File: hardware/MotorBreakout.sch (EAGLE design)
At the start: 1 part

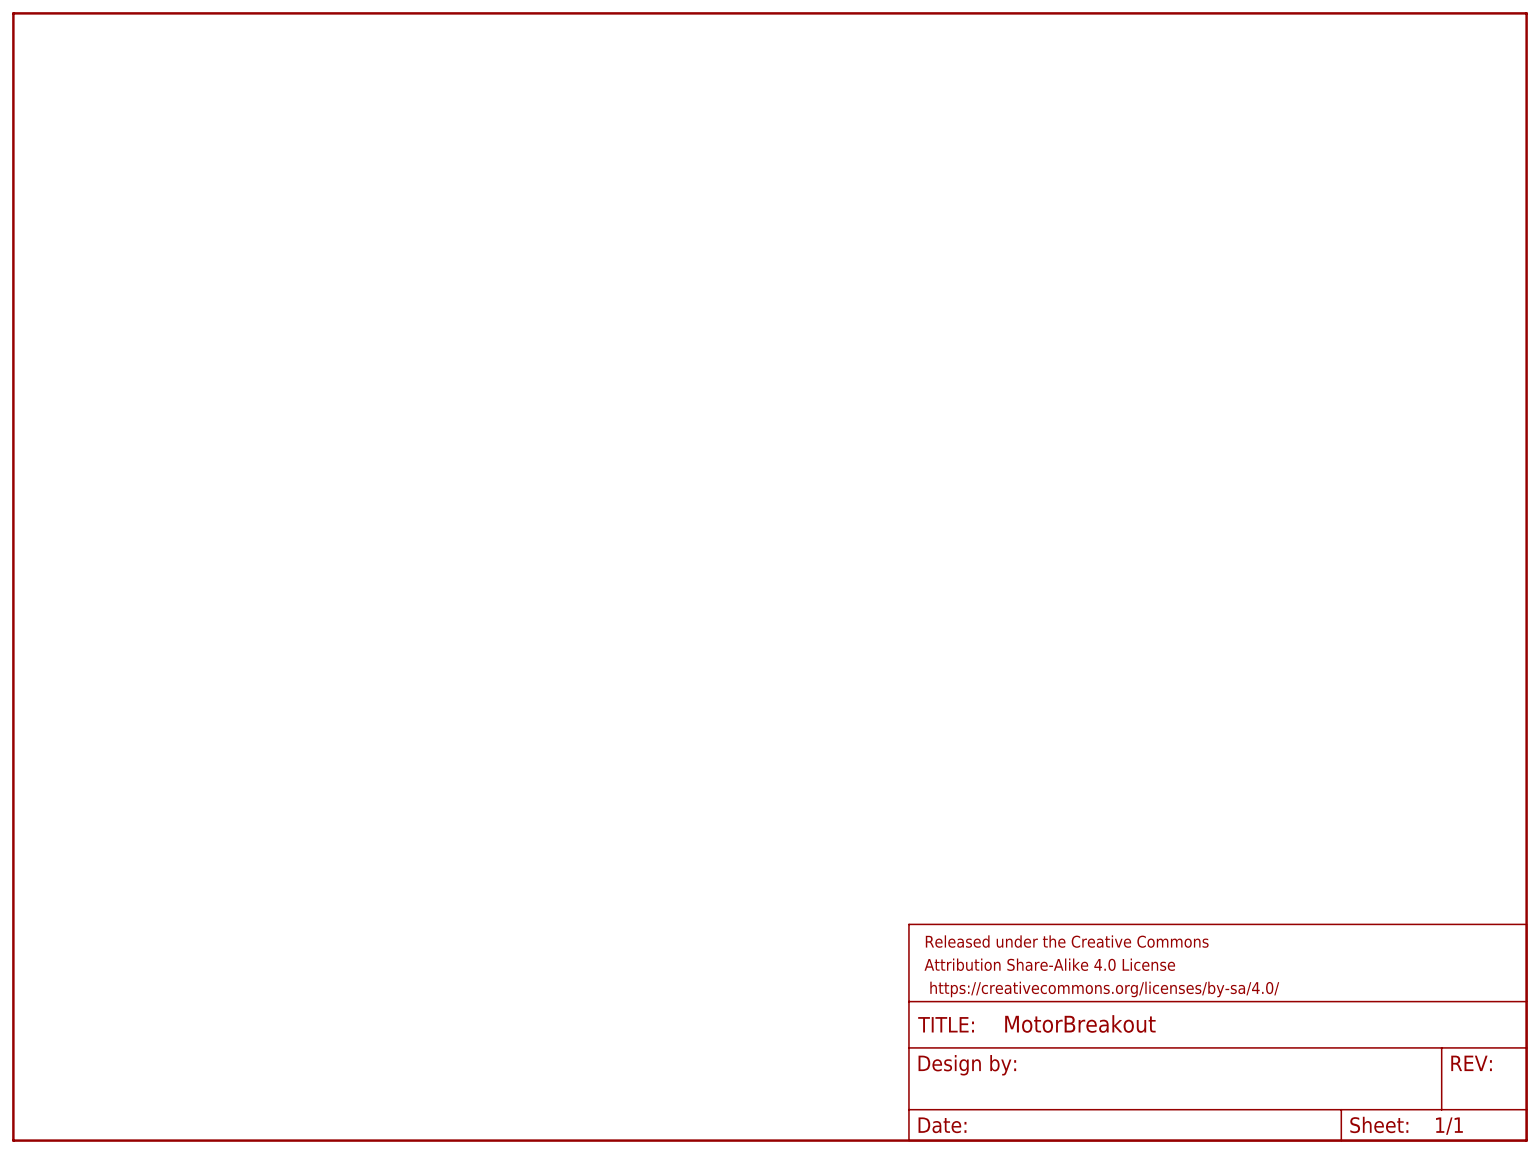
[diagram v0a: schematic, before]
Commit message: Basic breakout complete.y
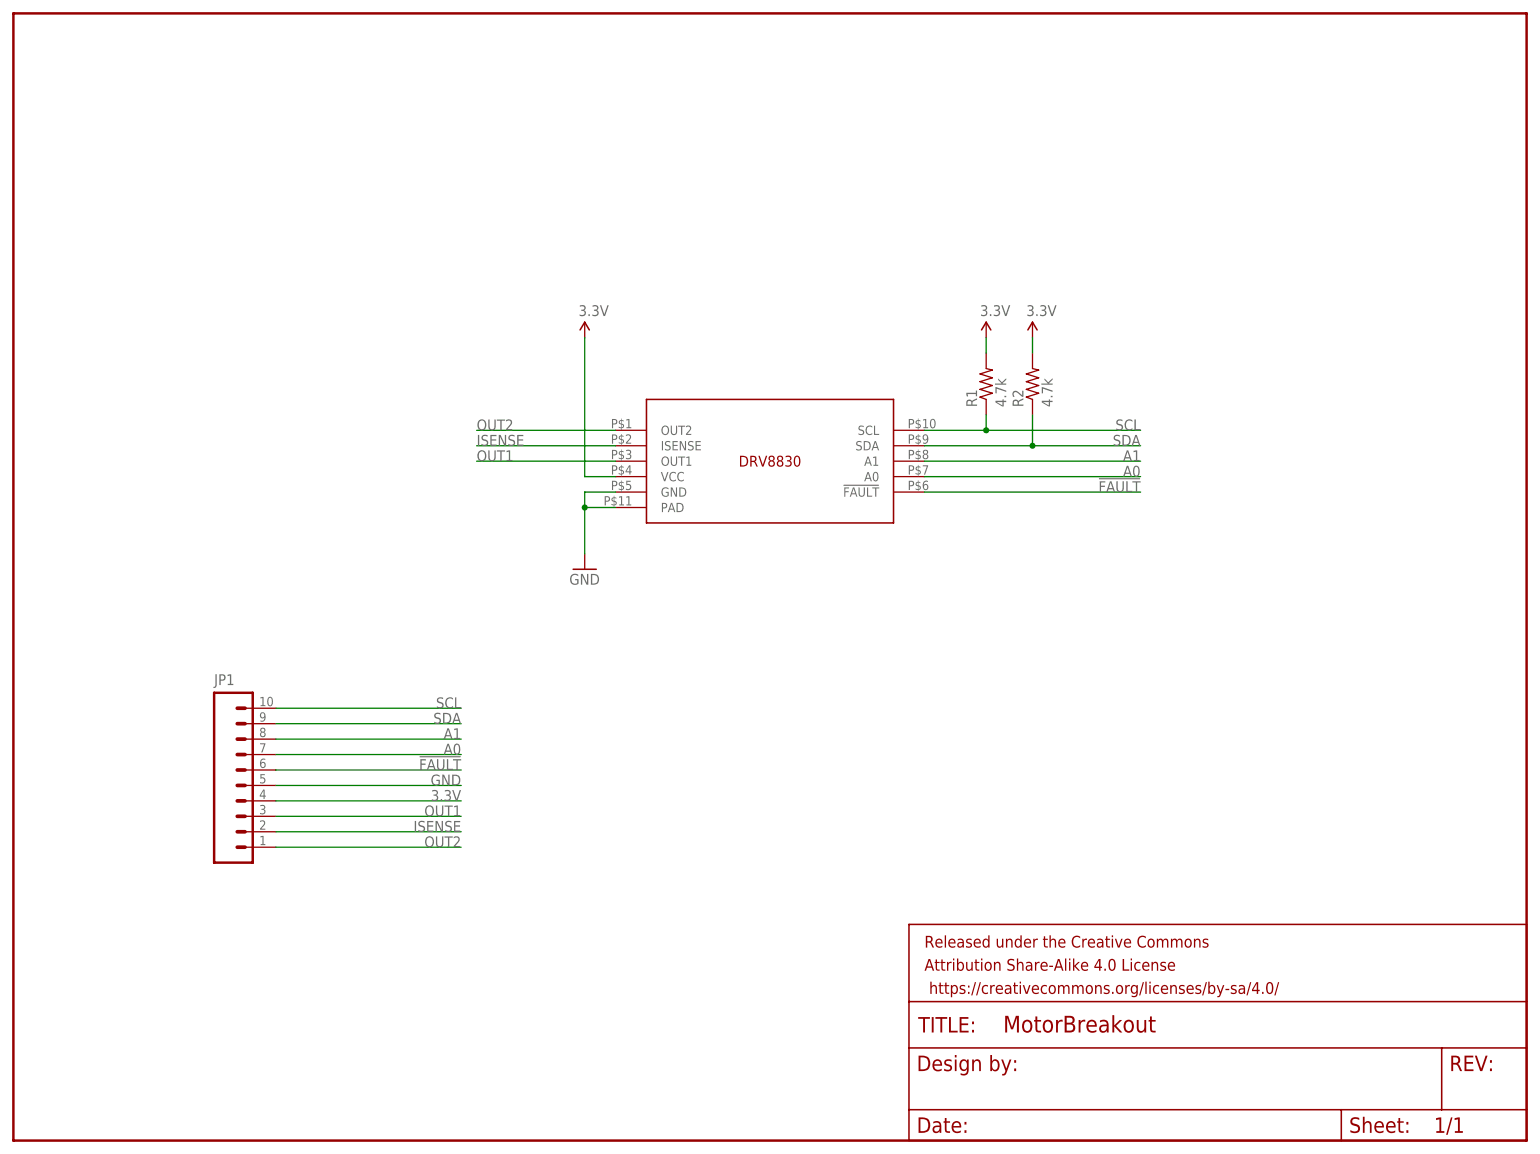
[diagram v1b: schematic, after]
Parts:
- added JP1: (no value), SparkFun-Connectors:M10LOCK_LONGPADS
- added R1, R2: 4.7k, SparkFun-Resistors:RESISTOR0402
- added U$1: DRV8830, DRV8830:DRV8830
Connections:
- new net !FAULT: JP1.6, U$1.!FAULT
- new net 3.3V: JP1.4, R1.2, R2.2, U$1.VCC
- new net A0: JP1.7, U$1.A0
- new net A1: JP1.8, U$1.A1
- new net GND: JP1.5, U$1.GND, U$1.PAD
- new net ISENSE: JP1.2, U$1.ISENSE
- new net OUT1: JP1.3, U$1.OUT1
- new net OUT2: JP1.1, U$1.OUT2
- new net SCL: JP1.10, R1.1, U$1.SCL
- new net SDA: JP1.9, R2.1, U$1.SDA
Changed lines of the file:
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@@
 <layer number="113" name="IDFDebug" color="4" fill="1" visible="yes" active="yes"/>
 <layer number="116" name="Patch_BOT" color="9" fill="4" visible="yes" active="yes"/>
+<layer number="118" name="Rect_Pads" color="7" fill="1" visible="yes" active="yes"/>
 <layer number="121" name="_tsilk" color="7" fill="1" visible="yes" active="yes"/>
 <layer number="122" name="_bsilk" color="7" fill="1" visible="yes" active="yes"/>
@@
 <parts>
 <part name="FRAME1" library="SparkFun-Aesthetics" deviceset="FRAME-LETTER" device="NO_PACKAGE"/>
+<part name="U$1" library="DRV8830" deviceset="DRV8830" device=""/>
+<part name="GND1" library="SparkFun-Aesthetics" deviceset="GND" device=""/>
+<part name="SUPPLY1" library="SparkFun-Aesthetics" deviceset="3.3V" device=""/>
+<part name="JP1" library="SparkFun-Connectors" deviceset="M10" device="LOCK_LONGPADS"/>
+<part name="SUPPLY2" library="SparkFun-Aesthetics" deviceset="3.3V" device=""/>
+<part name="SUPPLY3" library="SparkFun-Aesthetics" deviceset="3.3V" device=""/>
+<part name="R1" library="SparkFun-Resistors" deviceset="RESISTOR" device="0402" value="4.7k"/>
+<part name="R2" library="SparkFun-Resistors" deviceset="RESISTOR" device="0402" value="4.7k"/>
 </parts>
 <sheets>
@@
 <instance part="FRAME1" gate="G$1" x="0" y="0"/>
 <instance part="FRAME1" gate="V" x="147.32" y="0"/>
+<instance part="U$1" gate="G$1" x="124.46" y="111.76"/>
+<instance part="GND1" gate="1" x="93.98" y="93.98"/>
+<instance part="SUPPLY1" gate="G$1" x="93.98" y="132.08"/>
+<instance part="JP1" gate="G$1" x="33.02" y="66.04"/>
+<instance part="SUPPLY2" gate="G$1" x="160.02" y="132.08"/>
+<instance part="SUPPLY3" gate="G$1" x="167.64" y="132.08"/>
+<instance part="R1" gate="G$1" x="160.02" y="124.46" rot="R90"/>
+<instance part="R2" gate="G$1" x="167.64" y="124.46" rot="R90"/>
 </instances>
 <busses>
 </busses>
 <nets>
+<net name="3.3V" class="0">
+<segment>
+<pinref part="U$1" gate="G$1" pin="VCC"/>
+<pinref part="SUPPLY1" gate="G$1" pin="3.3V"/>
+<wire x1="99.06" y1="109.22" x2="93.98" y2="109.22" width="0.1524" layer="91"/>
+<wire x1="93.98" y1="109.22" x2="93.98" y2="132.08" width="0.1524" layer="91"/>
+</segment>
+<segment>
+<pinref part="JP1" gate="G$1" pin="4"/>
+<wire x1="43.18" y1="55.88" x2="73.66" y2="55.88" width="0.1524" layer="91"/>
+<label x="73.66" y="55.88" size="1.778" layer="95" rot="MR0"/>
+</segment>
+<segment>
+<pinref part="SUPPLY2" gate="G$1" pin="3.3V"/>
+<pinref part="R1" gate="G$1" pin="2"/>
+<wire x1="160.02" y1="132.08" x2="160.02" y2="129.54" width="0.1524" layer="91"/>
+</segment>
+<segment>
+<pinref part="SUPPLY3" gate="G$1" pin="3.3V"/>
+<pinref part="R2" gate="G$1" pin="2"/>
+<wire x1="167.64" y1="132.08" x2="167.64" y2="129.54" width="0.1524" layer="91"/>
+</segment>
+</net>
+<net name="GND" class="0">
+<segment>
+<pinref part="U$1" gate="G$1" pin="GND"/>
+<pinref part="GND1" gate="1" pin="GND"/>
+<wire x1="99.06" y1="106.68" x2="93.98" y2="106.68" width="0.1524" layer="91"/>
+<wire x1="93.98" y1="106.68" x2="93.98" y2="104.14" width="0.1524" layer="91"/>
+<pinref part="U$1" gate="G$1" pin="PAD"/>
+<wire x1="93.98" y1="104.14" x2="93.98" y2="96.52" width="0.1524" layer="91"/>
+<wire x1="99.06" y1="104.14" x2="93.98" y2="104.14" width="0.1524" layer="91"/>
+<junction x="93.98" y="104.14"/>
+</segment>
+<segment>
+<pinref part="JP1" gate="G$1" pin="5"/>
+<wire x1="43.18" y1="58.42" x2="73.66" y2="58.42" width="0.1524" layer="91"/>
+<label x="73.66" y="58.42" size="1.778" layer="95" rot="MR0"/>
+</segment>
+</net>
+<net name="OUT1" class="0">
+<segment>
+<pinref part="U$1" gate="G$1" pin="OUT1"/>
+<wire x1="99.06" y1="111.76" x2="76.2" y2="111.76" width="0.1524" layer="91"/>
+<label x="76.2" y="111.76" size="1.778" layer="95"/>
+</segment>
+<segment>
+<pinref part="JP1" gate="G$1" pin="3"/>
+<wire x1="43.18" y1="53.34" x2="73.66" y2="53.34" width="0.1524" layer="91"/>
+<label x="73.66" y="53.34" size="1.778" layer="95" rot="MR0"/>
+</segment>
+</net>
+<net name="ISENSE" class="0">
+<segment>
+<pinref part="U$1" gate="G$1" pin="ISENSE"/>
+<wire x1="99.06" y1="114.3" x2="76.2" y2="114.3" width="0.1524" layer="91"/>
+<label x="76.2" y="114.3" size="1.778" layer="95"/>
+</segment>
+<segment>
+<pinref part="JP1" gate="G$1" pin="2"/>
+<wire x1="43.18" y1="50.8" x2="73.66" y2="50.8" width="0.1524" layer="91"/>
+<label x="73.66" y="50.8" size="1.778" layer="95" rot="MR0"/>
+</segment>
+</net>
+<net name="OUT2" class="0">
+<segment>
+<pinref part="U$1" gate="G$1" pin="OUT2"/>
+<wire x1="99.06" y1="116.84" x2="76.2" y2="116.84" width="0.1524" layer="91"/>
+<label x="76.2" y="116.84" size="1.778" layer="95"/>
+</segment>
+<segment>
+<pinref part="JP1" gate="G$1" pin="1"/>
+<wire x1="43.18" y1="48.26" x2="73.66" y2="48.26" width="0.1524" layer="91"/>
+<label x="73.66" y="48.26" size="1.778" layer="95" rot="MR0"/>
+</segment>
+</net>
+<net name="SCL" class="0">
+<segment>
+<pinref part="U$1" gate="G$1" pin="SCL"/>
+<wire x1="149.86" y1="116.84" x2="160.02" y2="116.84" width="0.1524" layer="91"/>
+<label x="185.42" y="116.84" size="1.778" layer="95" rot="MR0"/>
+<pinref part="R1" gate="G$1" pin="1"/>
+<wire x1="160.02" y1="116.84" x2="185.42" y2="116.84" width="0.1524" layer="91"/>
+<wire x1="160.02" y1="119.38" x2="160.02" y2="116.84" width="0.1524" layer="91"/>
+<junction x="160.02" y="116.84"/>
+</segment>
+<segment>
+<pinref part="JP1" gate="G$1" pin="10"/>
+<wire x1="43.18" y1="71.12" x2="73.66" y2="71.12" width="0.1524" layer="91"/>
+<label x="73.66" y="71.12" size="1.778" layer="95" rot="MR0"/>
+</segment>
+</net>
+<net name="SDA" class="0">
+<segment>
+<pinref part="U$1" gate="G$1" pin="SDA"/>
+<wire x1="149.86" y1="114.3" x2="167.64" y2="114.3" width="0.1524" layer="91"/>
+<label x="185.42" y="114.3" size="1.778" layer="95" rot="MR0"/>
+<pinref part="R2" gate="G$1" pin="1"/>
+<wire x1="167.64" y1="114.3" x2="185.42" y2="114.3" width="0.1524" layer="91"/>
+<wire x1="167.64" y1="119.38" x2="167.64" y2="114.3" width="0.1524" layer="91"/>
+<junction x="167.64" y="114.3"/>
+</segment>
+<segment>
+<pinref part="JP1" gate="G$1" pin="9"/>
+<wire x1="43.18" y1="68.58" x2="73.66" y2="68.58" width="0.1524" layer="91"/>
+<label x="73.66" y="68.58" size="1.778" layer="95" rot="MR0"/>
+</segment>
+</net>
+<net name="A1" class="0">
+<segment>
+<pinref part="U$1" gate="G$1" pin="A1"/>
+<wire x1="149.86" y1="111.76" x2="185.42" y2="111.76" width="0.1524" layer="91"/>
+<label x="185.42" y="111.76" size="1.778" layer="95" rot="MR0"/>
+</segment>
+<segment>
+<pinref part="JP1" gate="G$1" pin="8"/>
+<wire x1="43.18" y1="66.04" x2="73.66" y2="66.04" width="0.1524" layer="91"/>
+<label x="73.66" y="66.04" size="1.778" layer="95" rot="MR0"/>
+</segment>
+</net>
+<net name="A0" class="0">
+<segment>
+<pinref part="U$1" gate="G$1" pin="A0"/>
+<wire x1="149.86" y1="109.22" x2="185.42" y2="109.22" width="0.1524" layer="91"/>
+<label x="185.42" y="109.22" size="1.778" layer="95" rot="MR0"/>
+</segment>
+<segment>
+<pinref part="JP1" gate="G$1" pin="7"/>
+<wire x1="43.18" y1="63.5" x2="73.66" y2="63.5" width="0.1524" layer="91"/>
+<label x="73.66" y="63.5" size="1.778" layer="95" rot="MR0"/>
+</segment>
+</net>
+<net name="!FAULT" class="0">
+<segment>
+<pinref part="U$1" gate="G$1" pin="!FAULT"/>
+<wire x1="149.86" y1="106.68" x2="185.42" y2="106.68" width="0.1524" layer="91"/>
+<label x="185.42" y="106.68" size="1.778" layer="95" rot="MR0"/>
+</segment>
+<segment>
+<pinref part="JP1" gate="G$1" pin="6"/>
+<wire x1="43.18" y1="60.96" x2="73.66" y2="60.96" width="0.1524" layer="91"/>
+<label x="73.66" y="60.96" size="1.778" layer="95" rot="MR0"/>
+</segment>
+</net>
 </nets>
 </sheet>
